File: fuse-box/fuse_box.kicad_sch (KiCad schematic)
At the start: 44 parts, among them J1 PWR, J3 Conn_02x05_Counter_Clockwise, U1 AP63200WU

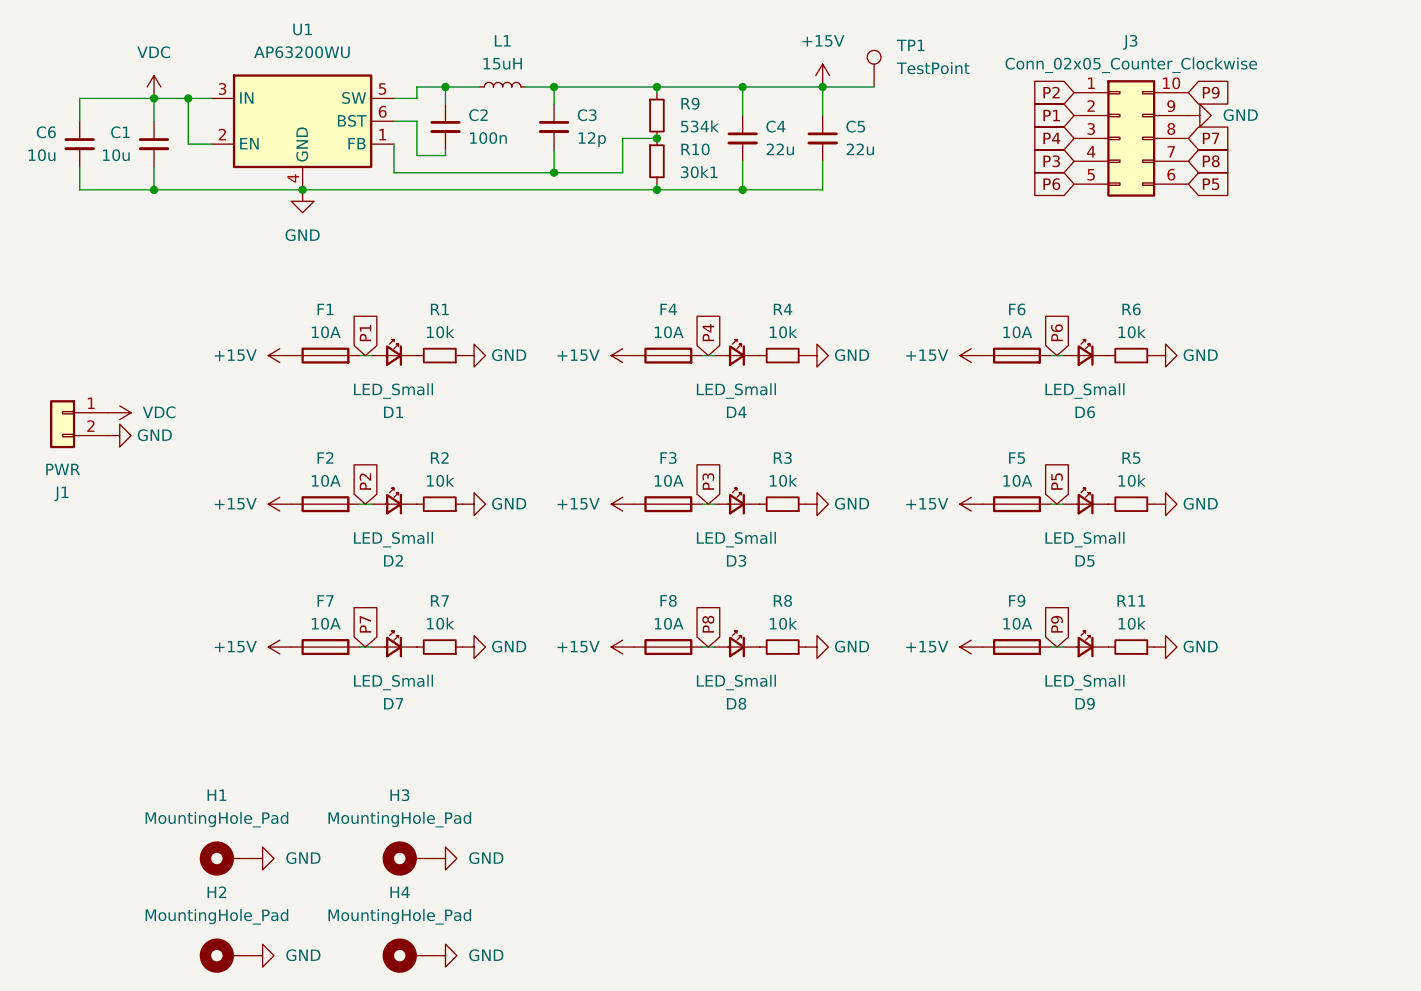
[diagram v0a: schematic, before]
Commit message: Add files via upload
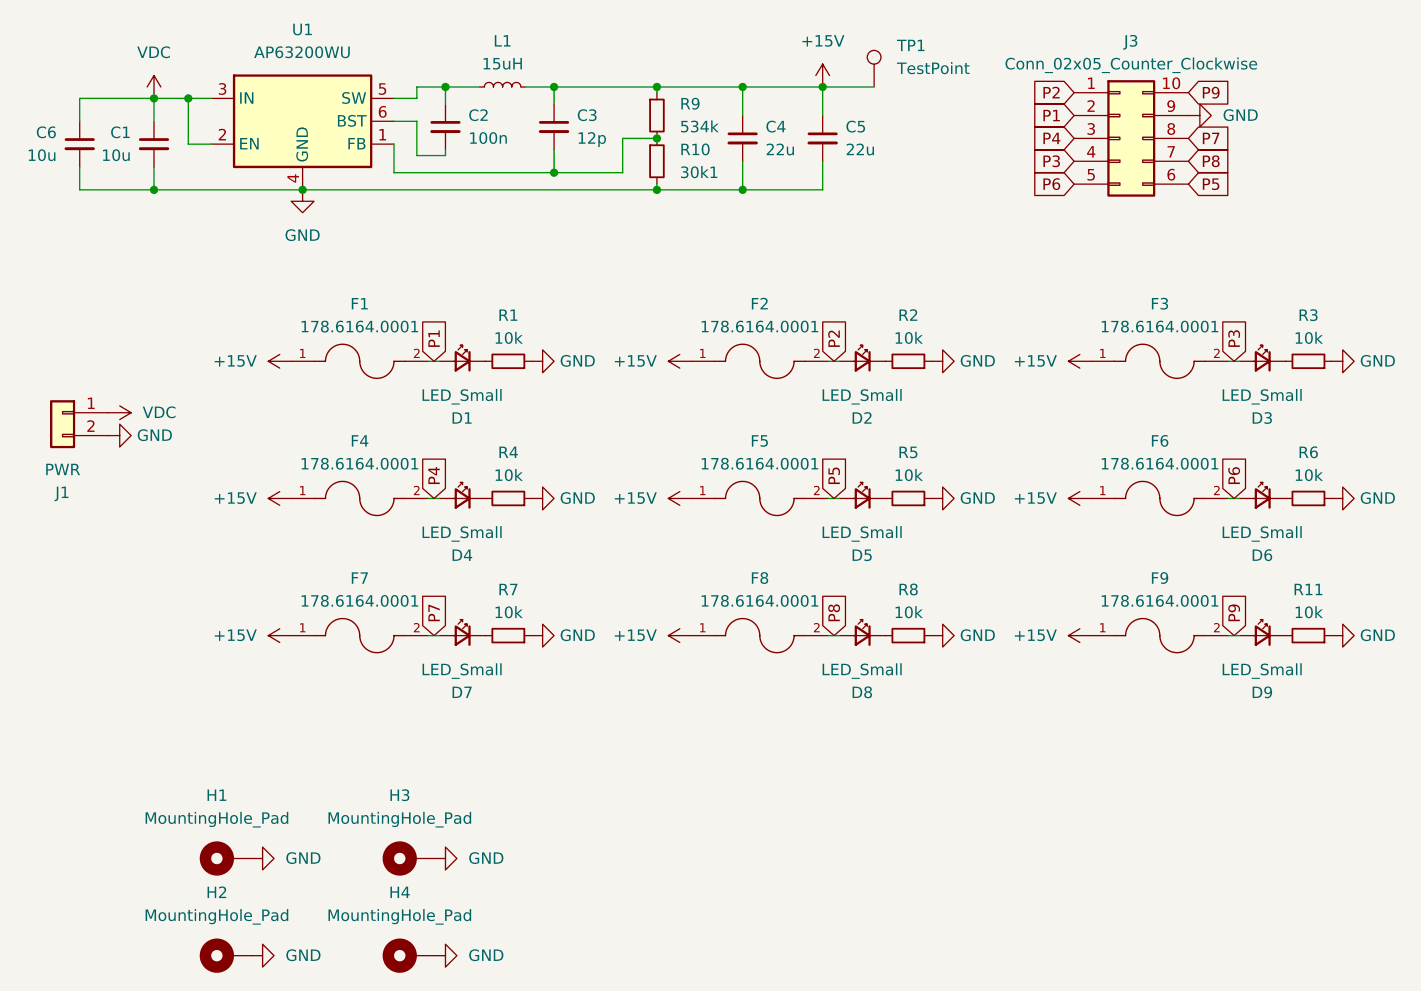
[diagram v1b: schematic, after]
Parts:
- removed F1, F2, F3, F4, F5, F6, F7, F8, F9: 10A, PCM_Fuse_AKL:Fuseholder_Blade_ATO_Littelfuse_Pudenz_2_Pin, symbol Device:Fuse
- added F1, F2, F3, F4, F5, F6, F7, F8, F9: 178.6164.0001, fuseholder:LITTELFUSE_178.6164.0001, symbol 178.6164.0001:178.6164.0001
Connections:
- net +15V: now also F1.1, F2.1, F3.1, F4.1, F5.1, F6.1, F7.1, F8.1, F9.1
- net P1: now also F1.2
- net P2: now also F2.2
- net P3: now also F3.2
- net P4: now also F4.2
- net P5: now also F5.2
- net P6: now also F6.2
- net P7: now also F7.2
- net P8: now also F8.2
- net P9: now also F9.2
